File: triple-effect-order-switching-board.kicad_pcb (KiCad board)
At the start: 4 copper layers, 138 x 86.5 mm, 4 parts, among them J1 Barrel_Jack_Switch, J2 AudioJack_TRS, J3 AudioJack_TRS

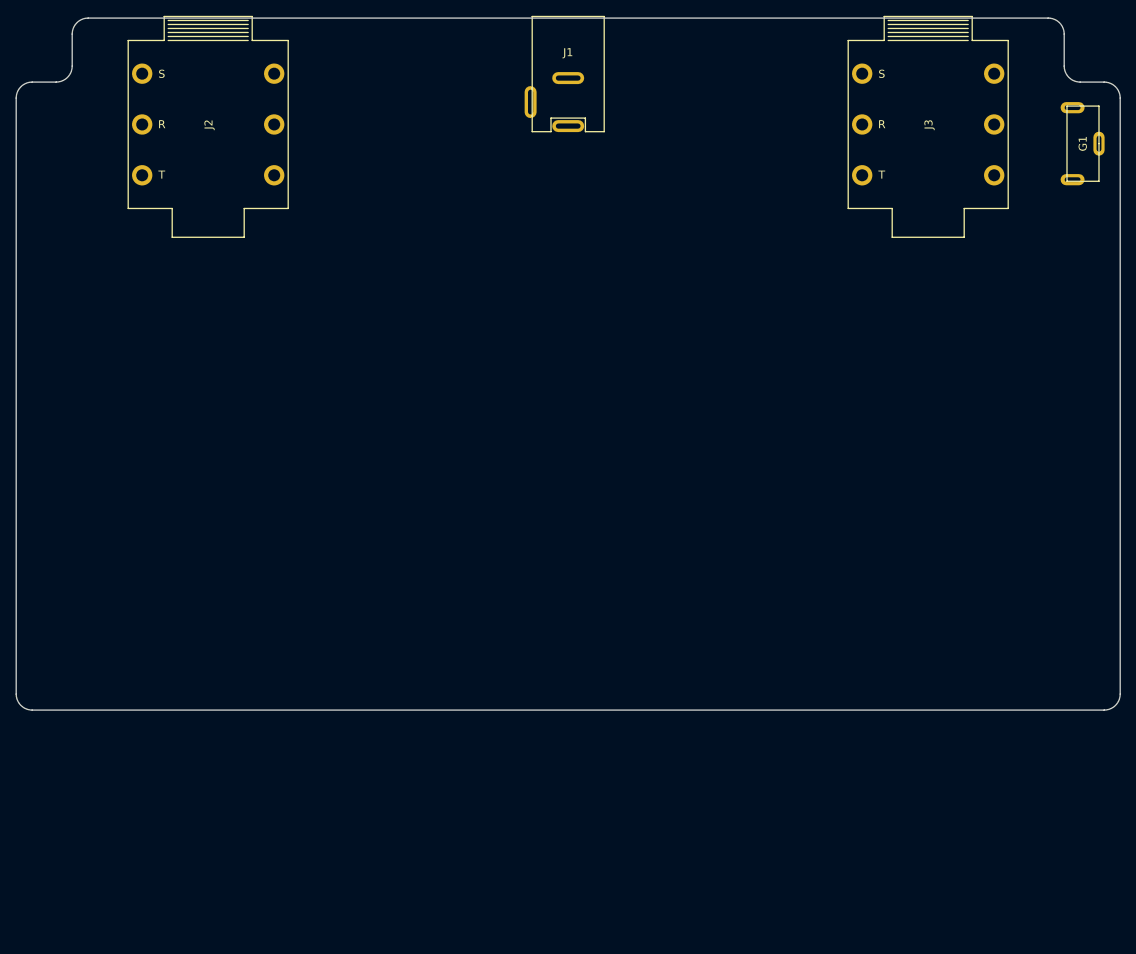
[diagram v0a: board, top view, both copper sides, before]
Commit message: finished board
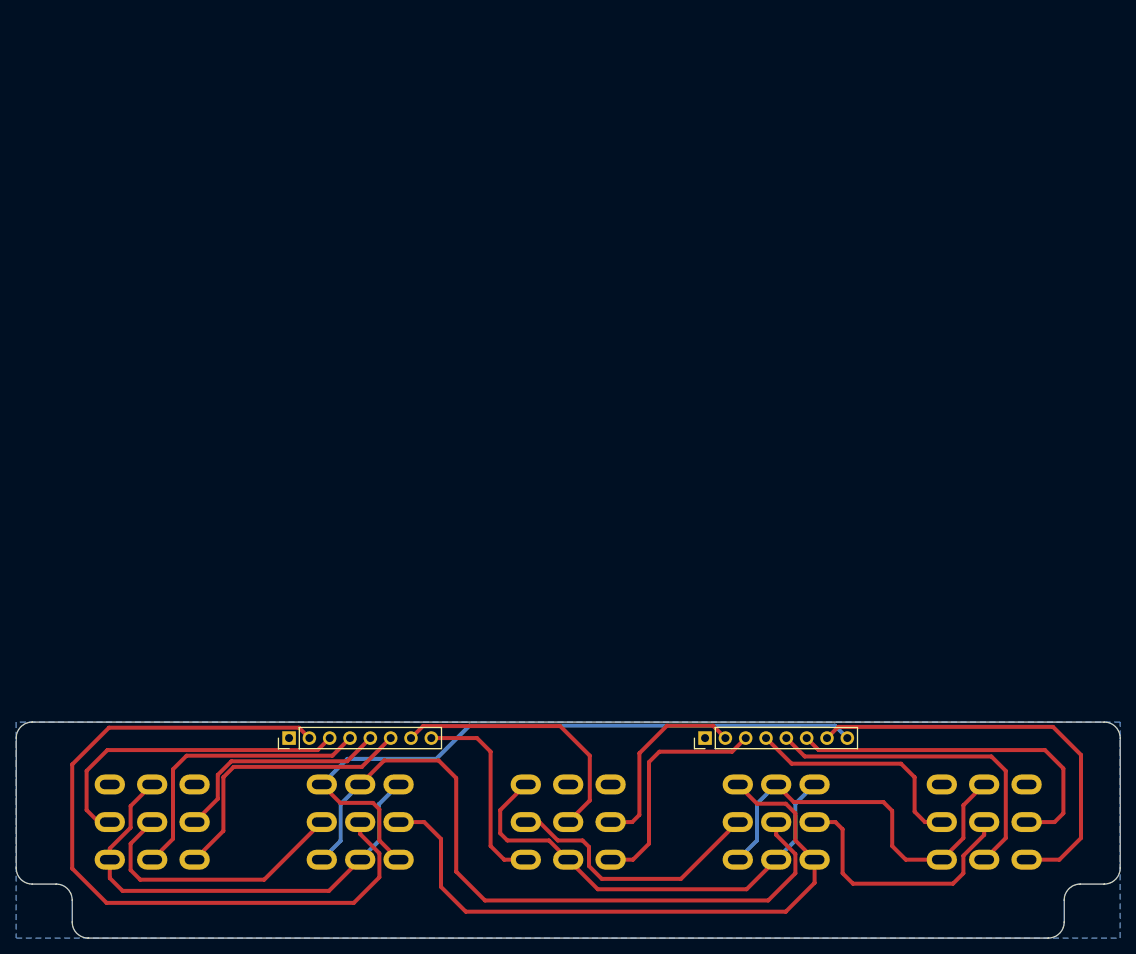
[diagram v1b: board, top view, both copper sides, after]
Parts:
- removed G1: GNDSpring, bca-footprints:Keystone_628
- removed J3: AudioJack_TRS, bca-footprints:Rean_NYS215
- added SW1: SW_3PDT, bca-footprints:SW_Toggle_3PDT_SolderLug, B.Cu at (26.0, 42.5)
- added SW2: SW_3PDT, bca-footprints:SW_Foot_3PDT, B.Cu at (-52.0, 42.5)
- added SW3: SW_3PDT, bca-footprints:SW_Foot_3PDT, B.Cu at (0.00, 42.5)
- added SW4: SW_3PDT, bca-footprints:SW_Foot_3PDT, B.Cu at (52.0, 42.5)
- added SW5: SW_3PDT, bca-footprints:SW_Toggle_3PDT_SolderLug, B.Cu at (-26.0, 42.5)
- J1: value Barrel_Jack_Switch -> Conn_01x08; footprint bca-footprints:DC_Jack_DC005 -> bca-footprints:Pin_Header_Straight_1x08_Pitch2.54mm
- J2: value AudioJack_TRS -> Conn_01x08; footprint bca-footprints:Rean_NYS215 -> bca-footprints:Pin_Header_Straight_1x08_Pitch2.54mm
- moved J2 104.5 mm to (26.0, 32.0)
- moved J1 93.9 mm to (-26.0, 32.0)
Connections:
- J1 pad 2: Net-(Q1-D) -> /input_jack
- J1 pad 3: unconnected-(J1-Pad3) -> /send0
- J2 pad 1: /input_jack -> Earth
- J2 pad 2: Earth -> /led1
- J2 pad 3: Earth -> /v1
- J2 pad 4: Earth -> /send2
- J2 pad 5: Earth -> /return2
- J2 pad 6: Earth -> /led2
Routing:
- net /input_jack: track 0.00 -> 94.5 mm
- net /os_in: track 0.00 -> 89.9 mm
- net /output_jack: track 0.00 -> 85.2 mm
- net /os_out: track 0.00 -> 80.0 mm
- net /in0: track 0.00 -> 58.9 mm
- net /in1: track 0.00 -> 57.7 mm
- net /v2: track 0.00 -> 52.1 mm
- net /in2: track 0.00 -> 50.2 mm
- net /led2: track 0.00 -> 44.3 mm
- net /return2: track 0.00 -> 41.3 mm
- net /send0: track 0.00 -> 40.5 mm
- net /return0: track 0.00 -> 36.1 mm
- net /v0: track 0.00 -> 34.7 mm
- net /out0: track 0.00 -> 34.5 mm
- net /send1: track 0.00 -> 33.9 mm
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- added copper zone on B.Cu, net Earth
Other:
- board size 138 x 86.5 mm -> 138 x 27 mm
- copper layers 4 -> 2
- board text removed: "JLCJLCJLCJLC"
